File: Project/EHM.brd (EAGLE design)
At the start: 78 x 60 mm, 116 parts, among them J1 282834-2, J2 282834-2, J3 282834-2, J4 282834-2, J5 282834-2, J6 S6B-PH-SM4-TB(LF)(SN), J7 S2B-PH-SM4-TB(LF)(SN), Q1 BC557B, Q2 BC547B, U1 BQ25570RGRR, U2 MAX9934TAUA, U3 MAX9934TAUA, U4 MAX9620, U5 MAX9620, U6 MAX9620

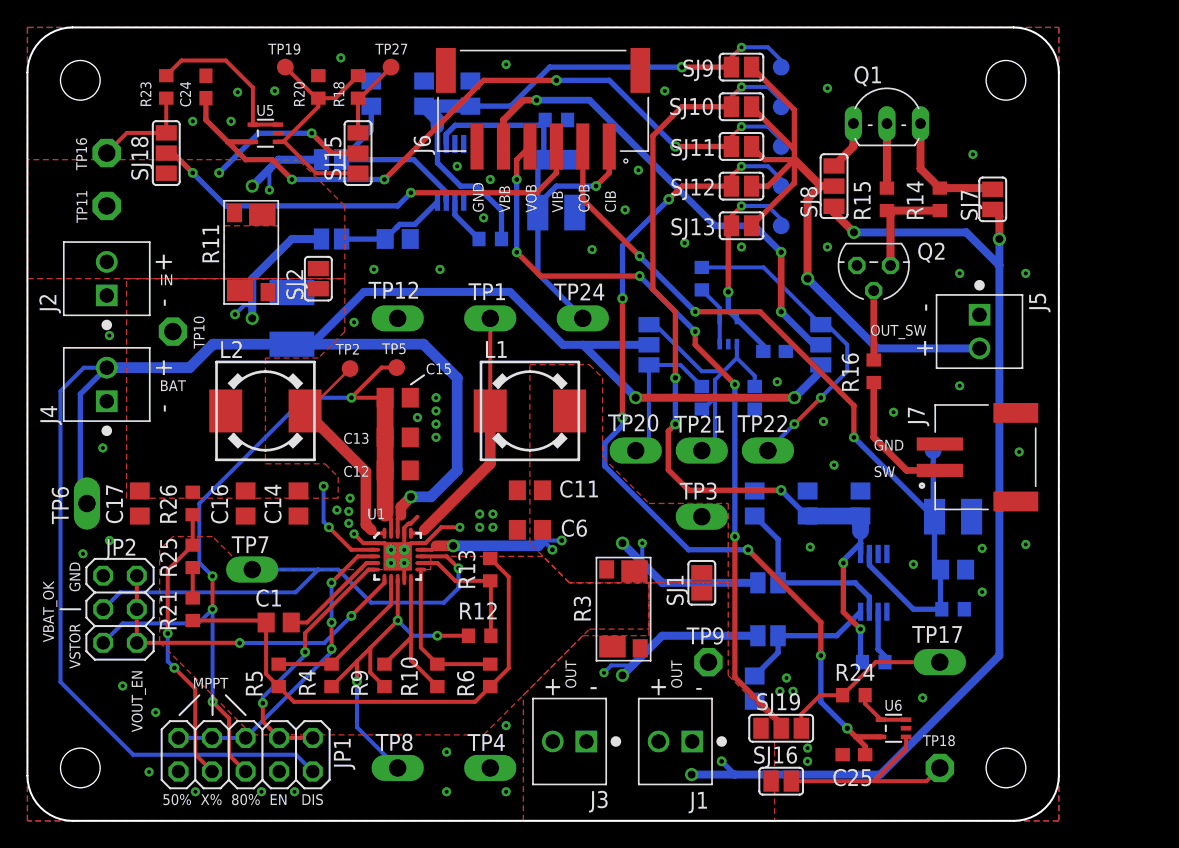
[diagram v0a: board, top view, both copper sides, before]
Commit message: First commit to develop branch
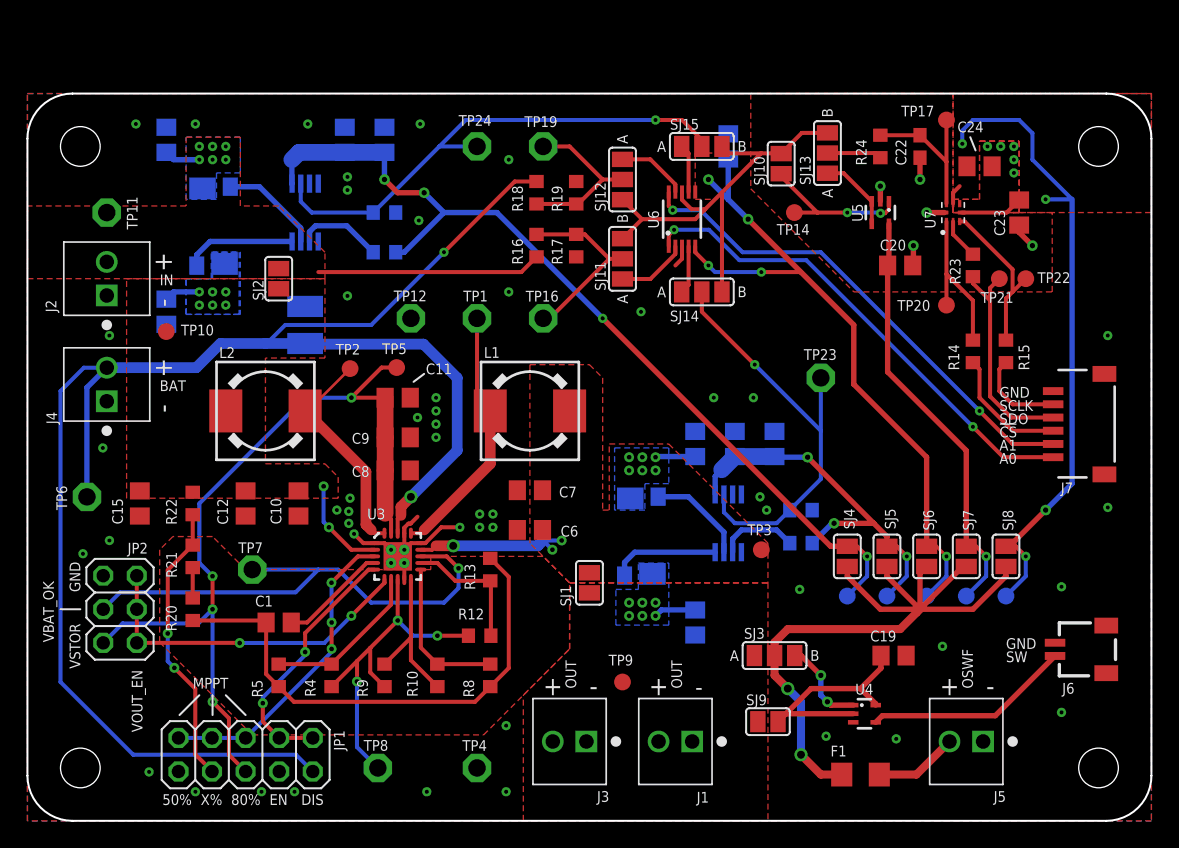
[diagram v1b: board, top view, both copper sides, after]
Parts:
- removed C25: 0.1uF, rcl:C0603
- removed Q1: BC557B, transistor-pnp:TO92-EBC
- removed Q2: BC547B, transistor-npn:TO92
- removed R25: 0R, rcl:R0603
- removed R26: 7.87M, rcl:R0603
- removed SJ16: (no value), jumper:SJ
- removed SJ17, SJ18, SJ19: (no value), jumper:SJ_2
- removed TP27: TPB1,27, testpad:B1,27
- added F1: 1206L012THR, 1206L012THR:R1206
- added U7: ADS7041IRUGR, ADS7041IRUG:QFN50P150X150X40-8N
- C12: value 0.1uF -> 4.7uF
- C13, C7: value 4.7uF -> DNP
- C14: value 0.1uF -> DNP
- C16: value 4.7uF -> 0.1uF
- C17, C19: value DNP -> 0.1uF
- C18: value DNP -> 100uF; device rcl:C0805 -> rcl:C1210
- C2: value DNP -> 4.7uF; device rcl:C1210 -> rcl:C0805
- C22: value DNP -> 1.5nF; device rcl:C1812 -> rcl:C0603
- C23, C24: value 0.1uF -> 1uF; device rcl:C0603 -> rcl:C0805
- C3: value DNP -> 0.1uF; device rcl:C1210 -> rcl:C0805
- C4: value 0.01uF -> 4.7uF
- C5: value 0.01uF -> 0.1uF
- J6: value S6B-PH-SM4-TB(LF)(SN) -> SM02B-SRSS-TB(LF)(SN); device S6B-PH-SM4-TB_LF__SN_:JST_S6B-PH-SM4-TB(LF)(SN) -> SM02B-SRSS-TB(LF)(SN):SM02B-SRSS-TB
- J7: value S2B-PH-SM4-TB(LF)(SN) -> SM06B-SRSS-TB(LF)(SN); device S2B-PH-SM4-TB_LF__SN_:JST_S2B-PH-SM4-TB(LF)(SN) -> SM06B-SRSS-TB(LF)(SN):SM06B-SRSS-B
- R14: value 10k -> 50R
- R15: value 2.2k -> 50R
- R16: value 18k -> 10M
- R20: value 10M -> 5.23M
- R21: value 5.23M -> 0R
- R22: value 0R -> 7.87M
- R23: value 0R -> 50R
- R24: value 0R -> 200R
- R6: value 5.11M -> 10k
- R8: value 10k -> 5.11M
- SJ11, SJ12, SJ13, SJ3: device jumper:SJ -> jumper:SJ_2
- SJ8: device jumper:SJ_2 -> jumper:SJ
- TP1, TP12, TP24, TP4, TP6, TP7, TP8: value TPPAD1-13Y -> TPPAD1-13; device testpad:P1-13Y -> testpad:P1-13
- TP10, TP18, TP9: value TPPAD1-13 -> TPB1,27; device testpad:P1-13 -> testpad:B1,27
- TP17, TP20, TP21, TP22, TP3: value TPPAD1-13Y -> TPB1,27; device testpad:P1-13Y -> testpad:B1,27
- TP19, TP23: value TPB1,27 -> TPPAD1-13; device testpad:B1,27 -> testpad:P1-13
- U1: value BQ25570RGRR -> MAX9934TAUA; device BQ25570RGRR:QFN50P350X350X100-21N -> MAX9934TAUA:21-0036K
- U3: value MAX9934TAUA -> BQ25570RGRR; device MAX9934TAUA:21-0036K -> BQ25570RGRR:QFN50P350X350X100-21N
- U4: value MAX9620 -> MAX4715; device MAX9620:SC70-5 -> MAX4715:SC70-5L
- U5: value MAX9620 -> OPA314IDCKR; device MAX9620:SC70-5 -> OPA314IDCK:SC70-5L
- U6: value MAX9620 -> DG2034EDQ-T1-GE3; device MAX9620:SC70-5 -> DG2034EDQ-T1-GE3:MSOP10
- moved R23 62.5 mm to (71.5, 42.0), turned to 90 degrees
- moved C24 58.8 mm to (72.0, 49.5), turned to 0 degrees
- moved J6 55.9 mm to (80.0, 13.0), turned to 90 degrees
- moved C3 54.1 mm to (24.0, 51.5), turned to 270 degrees
- moved SJ5 51.6 mm to (65.0, 20.0), flipped to the top, turned to 90 degrees
- moved SJ9 49.5 mm to (56.0, 7.50)
- moved C22 49.2 mm to (67.5, 51.0), flipped to the top
- moved U5 46.9 mm to (64.5, 46.0), turned to 180 degrees
- moved SJ3 46.0 mm to (56.5, 12.5), flipped to the top
- moved C10 42.5 mm to (20.5, 24.0), flipped to the top
- moved C17 42.2 mm to (50.5, 28.5), flipped to the bottom, turned to 90 degrees
- moved R22 42.1 mm to (12.5, 24.0), flipped to the top
- moved C20 42.1 mm to (66.0, 42.0), flipped to the top, turned to 0 degrees
- moved U6 41.7 mm to (49.5, 45.5), turned to 0 degrees
- moved R24 41.5 mm to (64.5, 51.0), turned to 270 degrees
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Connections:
- removed net N$1: C18.1, SJ3.1, U2.8
- removed net N$11: C19.1, SJ4.1, U3.8
- removed net N$14: SJ16.2, TP18.TP, U6.1
- removed net N$15: R22.1, U4.3, U4.4
- removed net N$16: R22.2, SJ17.3, TP22.TP
- removed net N$17: R17.2, R19.2, SJ14.1, TP21.TP, U4.1
- removed net N$18: R17.1, SJ14.3, TP20.TP
- removed net N$19: Q2.2, R16.1
- removed net N$20: Q1.B, R15.2
- removed net N$21: Q1.C, SJ8.3
- removed net N$23: Q1.E, R14.1, SJ7.2
- removed net N$25: Q2.3, R14.2, R15.1
- removed net N$26: R18.1, SJ15.3, TP27.TP
- removed net N$7 (its old number): R8.2, U3.6
- removed net RSN2_BUF: J6.4, SJ19.2
- removed net RSP1_BUF: J6.3, SJ18.2
- removed net VBAT_BUF: J6.5, SJ17.2
- new net !CS!: R14.1, TP20.TP, U7.1
- new net A0: J7.1, U6.1
- new net A1: J7.2, U6.10
- new net BUF_IN: SJ10.1, SJ11.1, SJ12.3, SJ13.1, SJ14.1, SJ15.3, U6.8
- new net BUF_OUT: R24.2, SJ13.2
- new net N$27: SJ13.3, U5.3, U5.4
- new net N$4: R6.2, U1.6
- new net RSP1_DIV: R16.1, R17.2, SJ11.2, TP16.TP
- new net S1: SJ11.3, U6.2
- new net S2: SJ12.1, U6.9
- new net S3: SJ14.3, U6.4
- new net S4: SJ15.1, U6.7
- new net SCLK: R15.1, TP22.TP, U7.3
- new net SDO: J7.4, R23.1, TP21.TP
- new net V+: C19.1, SJ9.1, U4.2, U4.5
- new net VBAT_DIV: R18.1, R19.2, SJ12.2, TP19.TP
- net CMES1: now also SJ15.2, U1.2; no longer C2.1, C4.1, J6.1, U2.2
- net CMES2: now also SJ14.2, U2.2; no longer C3.1, C5.1, J6.2, U3.2
- net GND: now also C10.2, C2.1, C22.1, C23.1, C3.1, C4.1, C5.1, C7.2, C8.2, C9.2, J6.2, J6.3, J6.4, J7.6, J7.7, J7.8, R17.1, R8.1, U1.3, U3.1, U3.15, U3.17, U3.21, U3.22, U3.23, U3.24, U3.25, U3.9, U4.3, U6.3, U7.5, U7.8; no longer C10.1, C2.2, C22.2, C23.2, C25.2, C3.2, C4.2, C5.2, C7.1, C8.1, C9.1, J6.6, J6.S1, J6.S2, J7.2, J7.S1, J7.S2, Q2.1, R21.1, R6.1, U1.1, U1.15, U1.17, U1.21, U1.22, U1.23, U1.24, U1.25, U1.9, U3.3, U4.2, U6.2
- net LBOOST: now also U3.20; no longer U1.20
- net LBUCK: now also U3.16; no longer U1.16
- net N$10: now also SJ3.3, U4.1; no longer C21.1, SJ6.1, U3.7
- net N$12: now also J7.5, R15.2; no longer R23.2, SJ18.3, TP16.TP
- net N$13: now also C22.2, R24.1, U7.7; no longer R24.2, SJ19.3
- net N$2: now also R20.2, R21.1; no longer R21.2, R25.1
- net N$3: now also R21.2, R22.1; no longer R25.2, R26.1
- net N$5: now also R23.2, U7.2; no longer R23.1, U5.3, U5.4
- net N$6: now also F1.2, J5.2; no longer C20.1, SJ5.1, U2.7
- net N$8: now also SJ10.2, TP14.TP; no longer R18.2, R20.2, SJ15.1, TP19.TP
- net N$9: now also J7.3, R14.2; no longer R24.1, U6.3, U6.4
- net NEN: now also U3.5; no longer U1.5
- net OK_HYST: now also U3.10; no longer U1.10
- net OK_PROG: now also R8.2, U3.11; no longer R6.2, U1.11
- net RSN2: now also C14.1, SJ3.1, SJ9.2, U2.8; no longer SJ16.1, SJ19.1, SJ4.2, SJ7.1, SJ8.1
- net RSP1: now also C16.1, R16.2, U1.7; no longer SJ15.2, SJ18.1, SJ5.2
- net SW: now also J6.1, U4.4; no longer J7.1, R16.2
- net VBAT: now also C18.1, R18.2, U3.18; no longer C22.1, SJ14.2, SJ17.1, U1.18
- net VBAT_OK: now also U3.13; no longer U1.13
- net VBAT_OV: now also U3.7; no longer U1.7
- net VCC_SW: now also F1.1, SJ3.2, SJ4.1, SJ5.1, SJ6.1, SJ7.1, SJ8.1; no longer J5.2, SJ10.1, SJ11.1, SJ12.1, SJ13.1, SJ8.2, SJ9.1
- net VCC_SW1: now also C2.2, C3.2, R6.1, SJ4.2, U1.1; no longer C7.2, C8.2, R7.1, SJ9.2, U2.1
- net VCC_SW2: now also C4.2, C5.2, R7.1, SJ5.2, U2.1; no longer C10.2, C9.2, R8.1, SJ10.2, U3.1
- net VCC_SW3: now also C21.1, SJ6.2, U6.5, U6.6; no longer C24.1, SJ11.2, U5.5
- net VCC_SW4: now also C20.1, SJ7.2, TP15.TP, U5.5; no longer C25.1, SJ12.2, TP14.TP, U6.5
- net VCC_SW5: now also C23.2, C24.1, SJ8.2, TP18.TP, U7.4, U7.6; no longer C23.1, SJ13.2, TP15.TP, U4.5
- net VIN_DC: now also C10.1, C12.1, C13.1, C15.1, R22.2, U1.8, U3.2; no longer C14.1, C16.1, C17.1, R26.2, SJ3.2, U1.2
- net VOC_SAMP: now also U3.3; no longer U1.3
- net VOUT: now also C17.1, C7.1, U2.7, U3.14; no longer C11.1, SJ6.2, U1.14
- net VOUT_EN: now also U3.6; no longer U1.6
- net VOUT_SET: now also U3.12; no longer U1.12
- net VRDIV: now also U3.8; no longer U1.8
- net VREF_SAMP: now also U3.4; no longer U1.4
- net VSTOR: now also C11.1, C8.1, C9.1, U3.19; no longer C12.1, C13.1, C15.1, U1.19
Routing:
- net RSN2: track 90.8 -> 11.4 mm
- net RSN2_BUF: track 57.1 -> 0.00 mm, vias 6 -> 0
- net VCC_SW5: track 16.4 -> 55.5 mm, vias 2 -> 4
- net VCC_SW2: track 67.8 -> 28.9 mm, vias 6 -> 3
- net A1: track 0.00 -> 37.6 mm, vias 0 -> 2
- net A0: track 0.00 -> 37.2 mm, vias 0 -> 2
- net VBAT_BUF: track 36.9 -> 0.00 mm, vias 3 -> 0
- net VCC_SW4: track 67.6 -> 32.3 mm, vias 7 -> 1
- net BUF_IN: track 0.00 -> 34.2 mm
- net RSP1_BUF: track 34.2 -> 0.00 mm, vias 2 -> 0
- net CMES2: track 61.9 -> 32.3 mm, vias 3 -> 1
- net VBAT: track 153.5 -> 126.0 mm, vias 3 -> 2
- net VCC_SW1: track 43.4 -> 67.9 mm, vias 2 -> 4
- net N$16: track 23.9 -> 0.00 mm, vias 2 -> 0
- net N$17: track 20.3 -> 0.00 mm
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- added copper zone on layer 1, net N$14
- added copper zone on layer 16, net RSN2
- added copper zone on layer 16, net RSP1
- added copper zone on layer 1, net VCC_SW3
- added copper zone on layer 1, net VCC_SW5
- added copper zone on layer 16, net VIN_DC
- added copper zone on layer 16, net VOUT
- removed copper zone on layer 1, net N$24
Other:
- board size 78 x 60 mm -> 85 x 55 mm
- board text added: "!CS!"
- board text added: "A"
- board text added: "A0"
- board text added: "A1"
- board text added: "B"
- board text added: "Energy Harvesting Monitor V2.0"
- board text added: "OSWF"
- board text added: "SCLK"
- board text added: "SDO"
- board text removed: "CIB"
- board text removed: "COB"
- board text removed: "Energy Harvesting Monitor V1.4"
- board text removed: "OUT_SW"
- board text removed: "VBB"
- board text removed: "VIB"
- board text removed: "VOB"
